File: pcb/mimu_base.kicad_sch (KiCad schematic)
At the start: 17 parts, among them J1 OPT, Q1 BSS84, SW1 SW_Push, SW2 In case mosfet does not work 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, U1 NSL-32SR3, U2 ATTINY88AU, U4 AD5258 - 1k

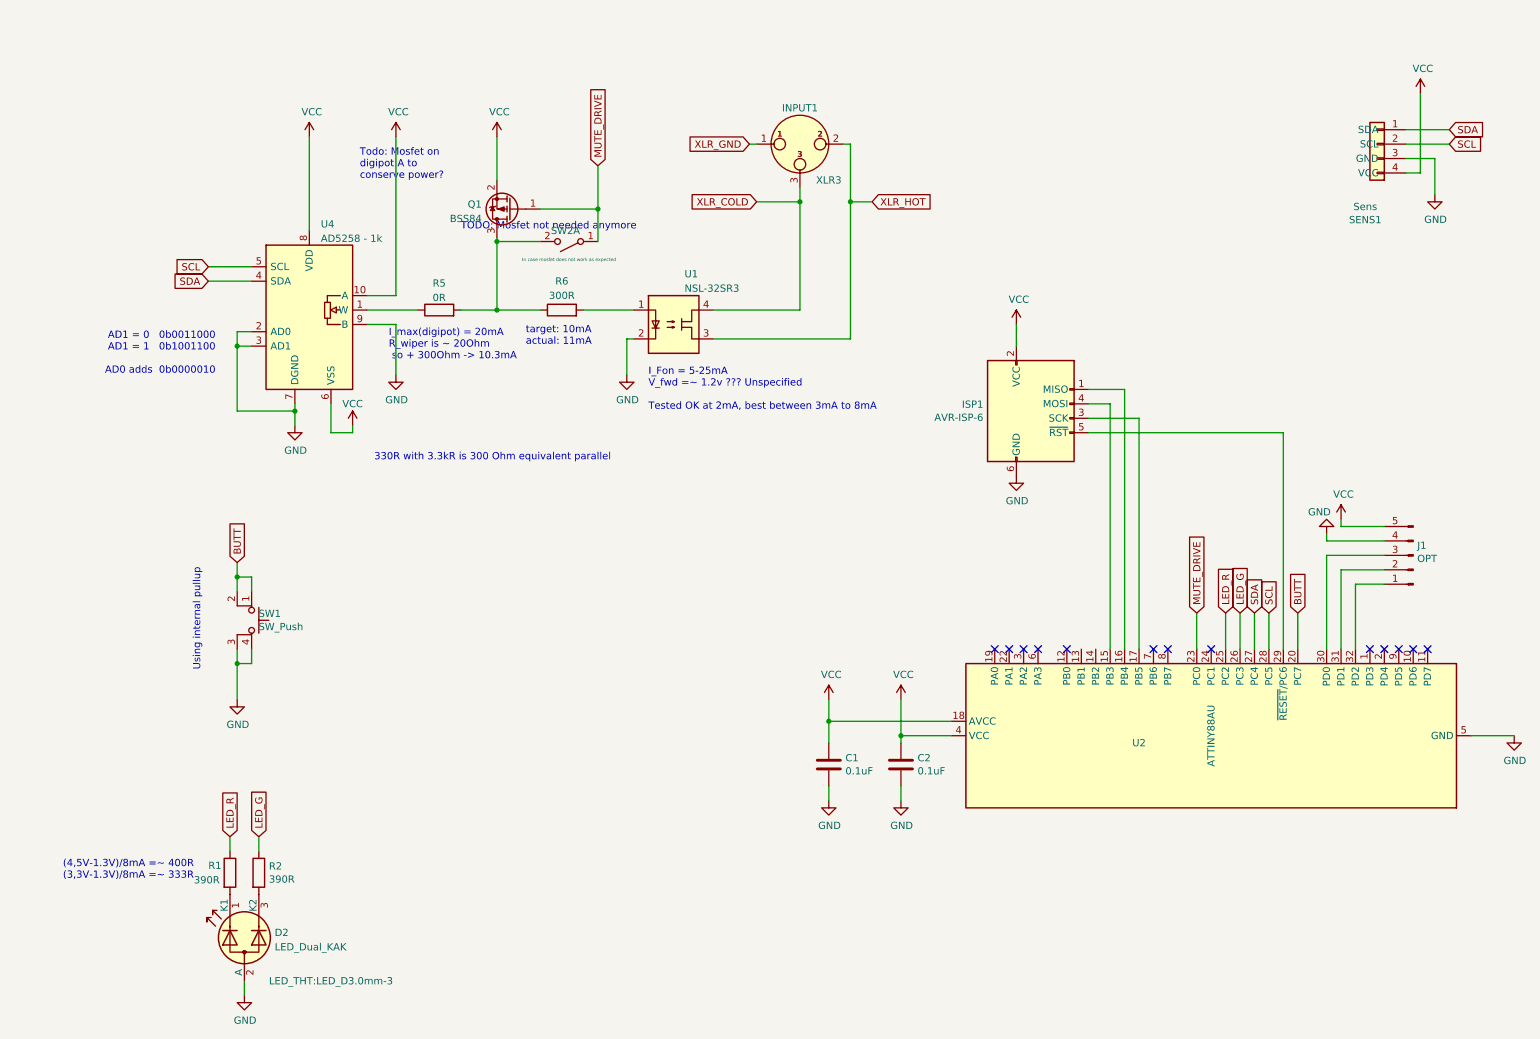
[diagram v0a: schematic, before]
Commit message: Initial playarounds for rheostat mode
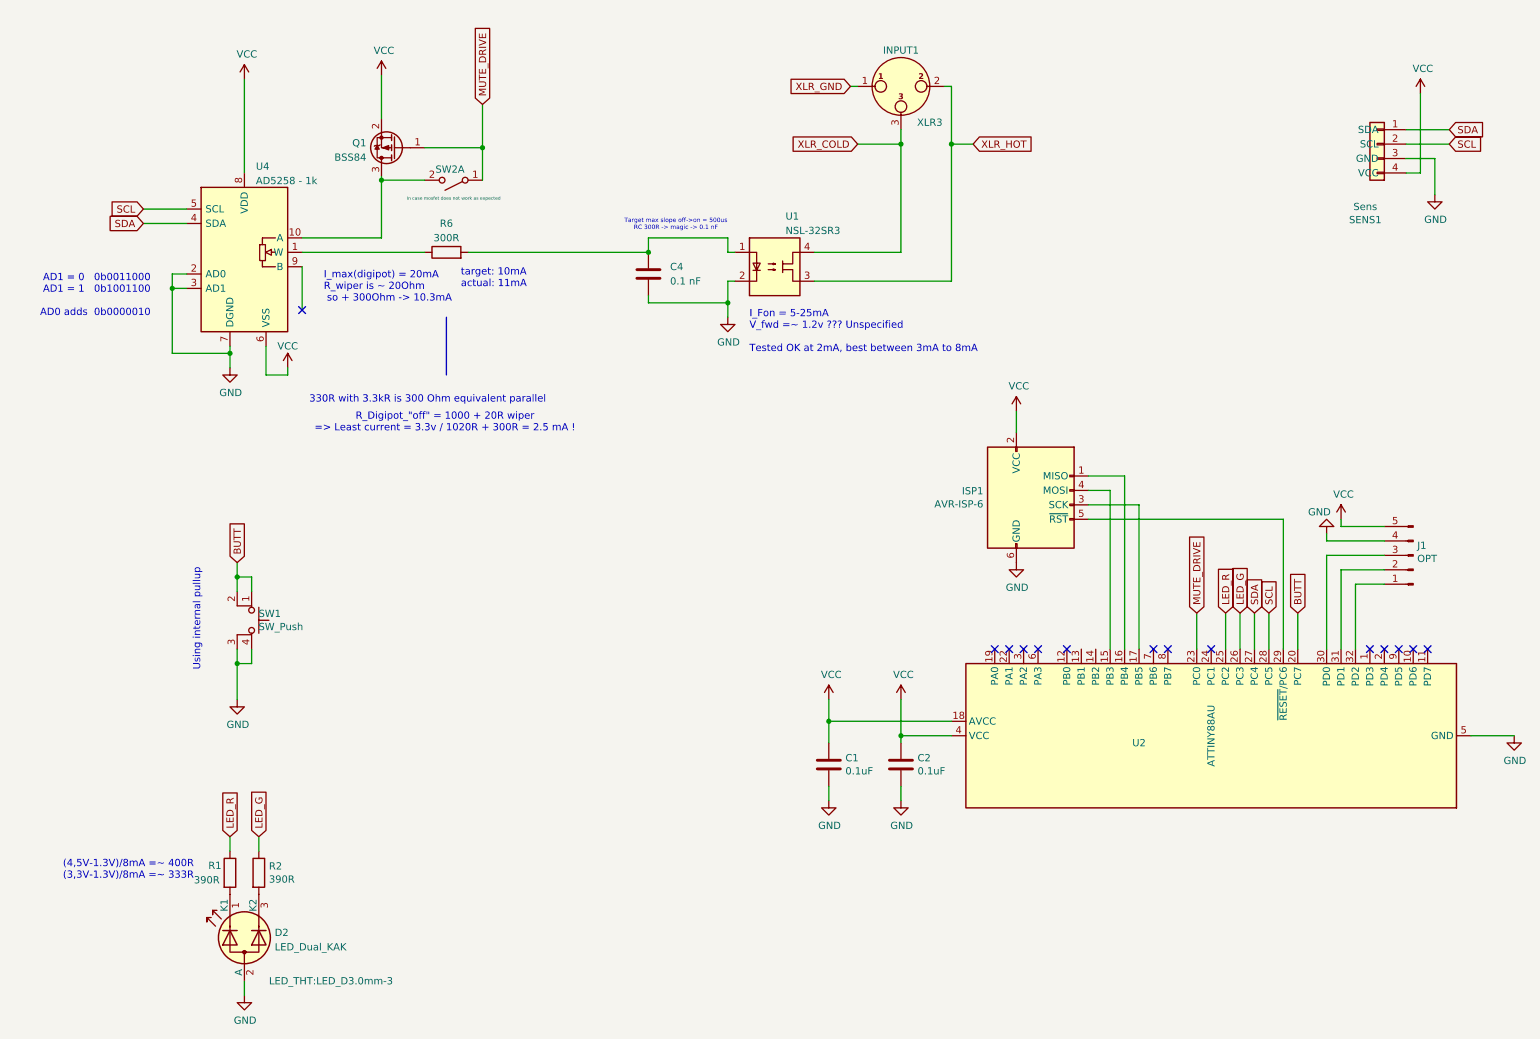
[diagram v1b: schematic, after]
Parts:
- removed R5: 0R, Resistor_SMD:R_1206_3216Metric_Pad1.30x1.75mm_HandSolder, symbol Device:R
- added C4: 0.1 nF, Resistor_SMD:R_1206_3216Metric_Pad1.30x1.75mm_HandSolder, symbol Device:C
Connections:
- net GND: now also C4.2; no longer U4.9 (B)
- net VCC: no longer U4.10 (A)
- net at R6.2, U1.1: now also C4.1
- net at Q1.3 (D), SW2.2 (B): now also U4.10 (A); no longer R6.1
- net at U4.1 (W): now also R6.1
- no-connect marks 13 -> 14
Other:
- note added: "R_Digipot_"off" = 1000 + 20R wiper => Least current = 3.3v / 1020R + 300R = 2.5 mA !"
- note added: "Target max slope off->on = 500us RC 300R -> magic -> 0.1 nF"
- note removed: "TODO: Mosfet not needed anymore"
- note removed: "Todo: Mosfet on digipot:A to conserve power?"
- moved on the sheet: INPUT1, ISP1, Q1, R6, SW2A, U1, U4
